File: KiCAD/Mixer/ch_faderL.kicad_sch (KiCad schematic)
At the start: 4 parts, among them U4 NE5532

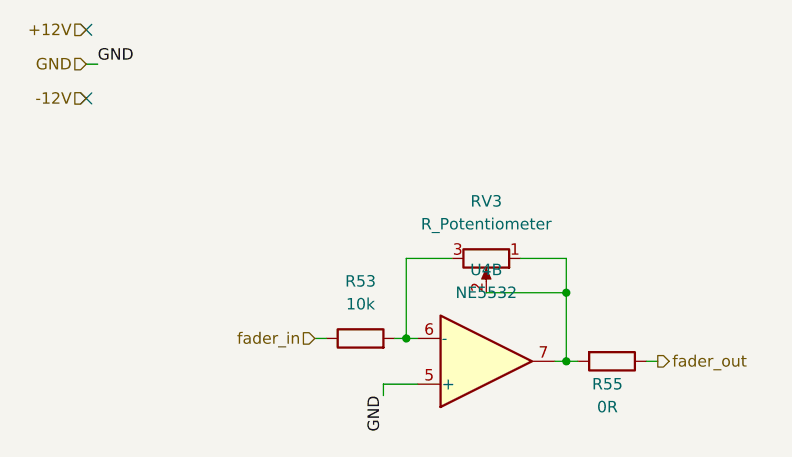
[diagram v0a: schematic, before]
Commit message: Final PCB Version that got ordered from JLCPCB
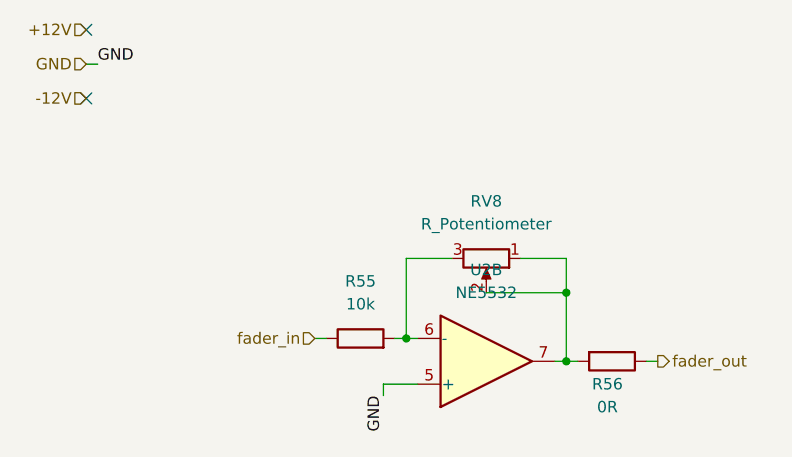
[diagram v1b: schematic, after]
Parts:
- removed R53: 10k, Resistor_SMD:R_0805_2012Metric_Pad1.20x1.40mm_HandSolder, symbol Device:R
- added R56: 0R, Resistor_SMD:R_0805_2012Metric_Pad1.20x1.40mm_HandSolder, symbol Device:R
- R55: value 0R -> 10k
- renumbered RV3 to RV8, U4 to U2
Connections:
- net fader_in: now also R55.1
- net fader_out: now also R56.1; no longer R55.1
- net at RV8.3, U2.6 (-): now also R55.2
- net at RV8.1, RV8.2, U2.7: now also R56.2; no longer R55.2
